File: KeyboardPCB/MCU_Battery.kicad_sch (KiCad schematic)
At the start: 23 parts, among them U1 ATmega32U4-M, U2 TPS61222DCK, U3 MCP73831-2-OT, Y1 ECS-160-7-33B-CKL-TR

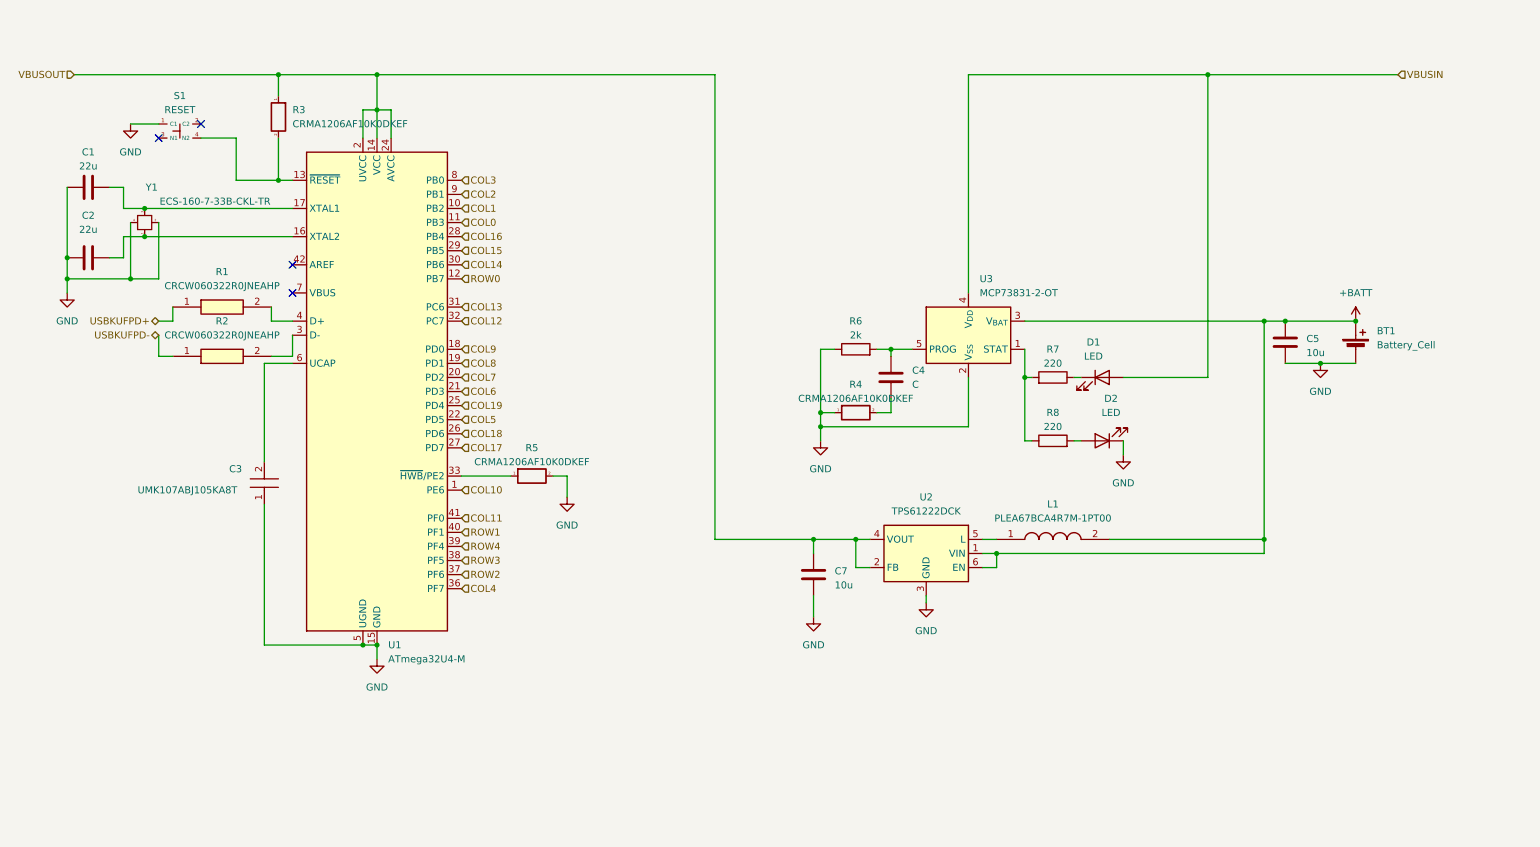
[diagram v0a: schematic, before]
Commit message: changed several components
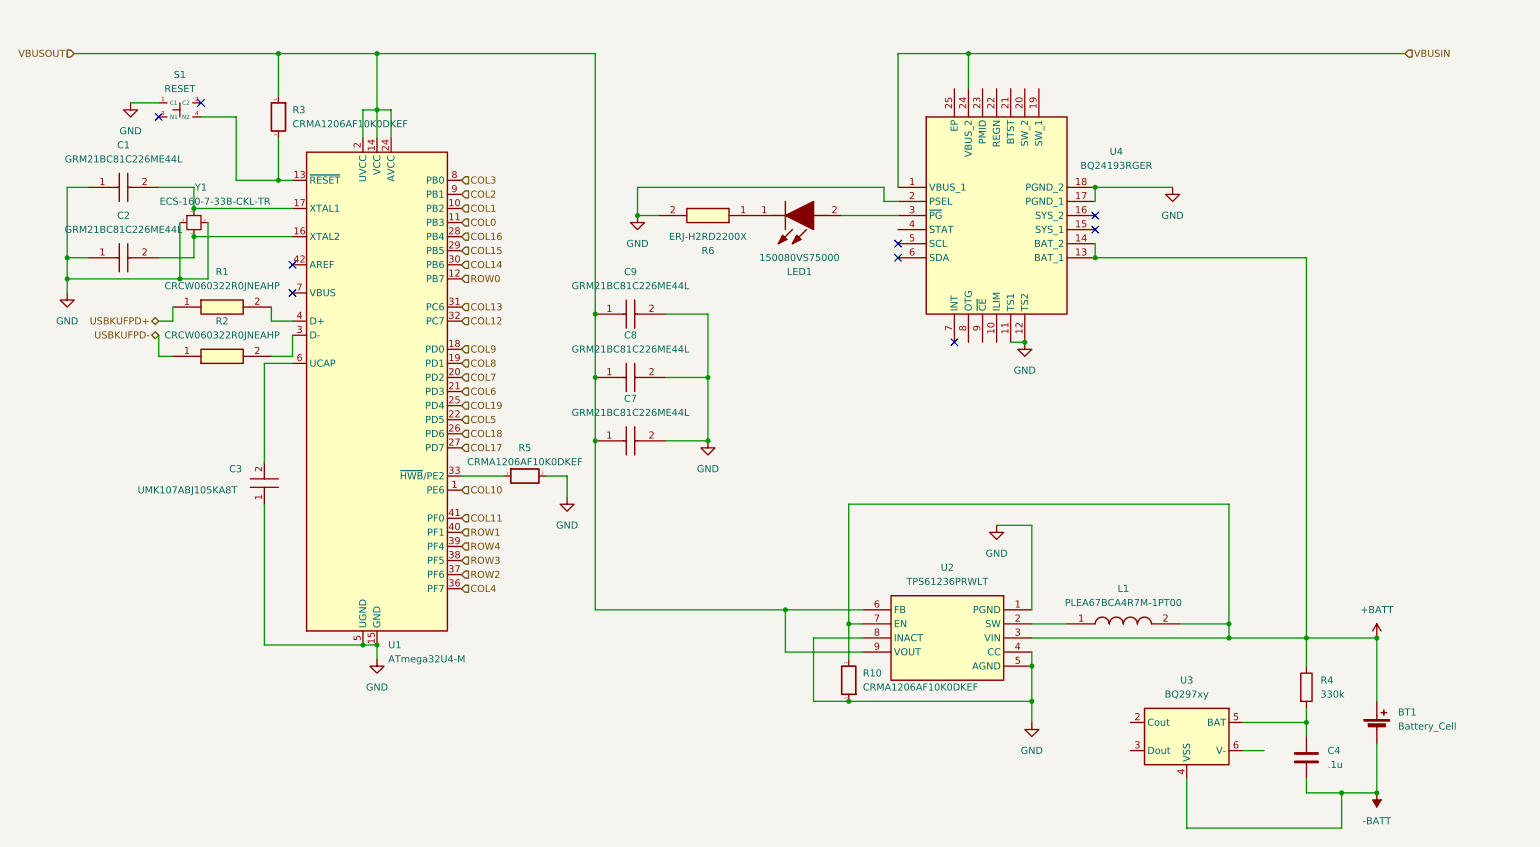
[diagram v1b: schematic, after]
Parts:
- removed C1, C2: 22u, symbol Device:C
- removed C5, C7: 10u, symbol Device:C
- removed D1, D2: LED, symbol Device:LED
- removed R4: CRMA1206AF10K0DKEF, keyboard_syms:RESC3216X74N, symbol keyboard_syms:CRMA1206AF10K0DKEF
- removed R6: 2k, symbol Device:R
- removed R7, R8: 220, symbol Device:R
- removed U2: TPS61222DCK, Package_TO_SOT_SMD:Texas_R-PDSO-G6, symbol Regulator_Switching:TPS61222DCK
- removed U3: MCP73831-2-OT, Package_TO_SOT_SMD:SOT-23-5, symbol Battery_Management:MCP73831-2-OT
- added C1, C2, C7, C8, C9: GRM21BC81C226ME44L, keyboard_syms:CAPC2012X145N, symbol keyboard_syms:GRM21BC81C226ME44L
- added LED1: 150080VS75000, keyboard_syms:LEDC2012X80N, symbol keyboard_syms:150080VS75000
- added R10: CRMA1206AF10K0DKEF, keyboard_syms:RESC3216X74N, symbol keyboard_syms:CRMA1206AF10K0DKEF
- added R4: 330k, symbol Device:R
- added R6: ERJ-H2RD2200X, keyboard_syms:H2C_H2R, symbol keyboard_syms:ERJ-H2RD2200X
- added U2: TPS61236PRWLT, keyboard_syms:TPS61235PRWLT, symbol keyboard_syms:TPS61236PRWLT
- added U3: BQ297xy, Package_SON:WSON-6_1.5x1.5mm_P0.5mm, symbol Battery_Management:BQ297xy
- added U4: BQ24193RGER, keyboard_syms:QFN50P400X400X100-25N-D, symbol keyboard_syms:BQ24193RGER
- C4: value C -> .1u
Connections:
- net +BATT: now also R10.2, R4.1, U2.3 (VIN), U2.7 (EN), U4.13 (BAT_1), U4.14 (BAT_2)
- net GND: now also C1.1, C2.1, C7.2, C8.2, C9.2, R10.1, R6.2, U2.1 (PGND), U2.4 (CC), U2.5 (AGND), U2.8 (INACT), U4.11 (TS1), U4.12 (TS2), U4.17 (PGND_1), U4.18 (PGND_2), U4.2 (PSEL); no longer BT1.2 (-)
- net VBUSIN: now also U4.1 (VBUS_1), U4.24 (VBUS_2)
- net VBUSOUT: now also C7.1, C8.1, C9.1, U2.6 (FB), U2.9 (VOUT)
- net at C4.1: now also R4.2, U3.5 (BAT)
- net -BATT: now reaches C4.2
- net -BATT: now also BT1.2 (-), U3.4 (VSS)
- net at U1.16 (XTAL2), Y1.1: now also C2.2
- net at U1.17 (XTAL1), Y1.3: now also C1.2
- net at L1.1: now also U2.2 (SW)
- new net: LED1.1 (K), R6.1
- new net: LED1.2 (A), U4.3 (~{PG})
- no-connect marks 4 -> 9
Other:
- moved on the sheet: R5, S1, Y1

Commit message: made changes to the board
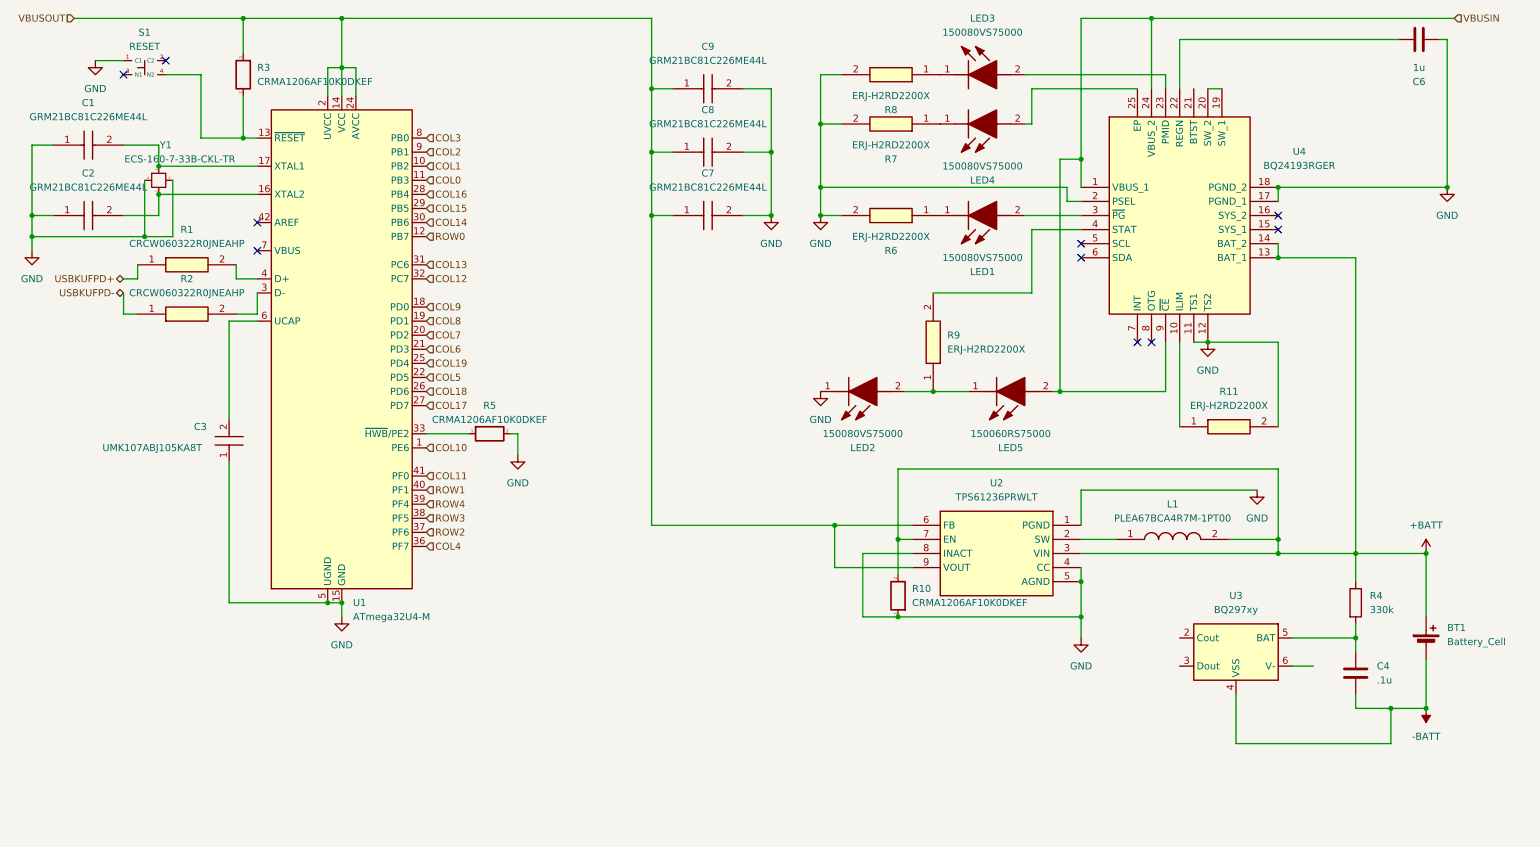
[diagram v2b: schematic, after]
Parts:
- added C6: 1u, symbol Device:C
- added LED2, LED3, LED4: 150080VS75000, keyboard_syms:LEDC2012X80N, symbol keyboard_syms:150080VS75000
- added LED5: 150060RS75000, keyboard_syms:LEDC1608X80N, symbol keyboard_syms:150060RS75000
- added R11, R7, R8, R9: ERJ-H2RD2200X, keyboard_syms:H2C_H2R, symbol keyboard_syms:ERJ-H2RD2200X
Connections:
- net GND: now also C6.2, LED2.1 (K), R11.2, R7.2, R8.2
- net VBUSIN: now also U4.9 (~{CE}), LED5.2 (A)
- net at U4.10 (ILIM): now also R11.1
- net at U4.19 (SW_1): now also U4.20 (SW_2)
- net at U4.22 (REGN): now also C6.1
- net at U4.23 (PMID): now also LED3.2 (A)
- net at U4.25 (EP): now also LED4.2 (A)
- net at U4.4 (STAT): now also R9.2
- new net: LED4.1 (K), R7.1
- new net: LED3.1 (K), R8.1
- new net: LED2.2 (A), LED5.1 (K), R9.1
- no-connect marks 9 -> 10
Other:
- moved on the sheet: BT1, C1, C2, C3, C4, C7, C8, C9, L1, LED1, R1, R10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

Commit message: Schematic Filled out
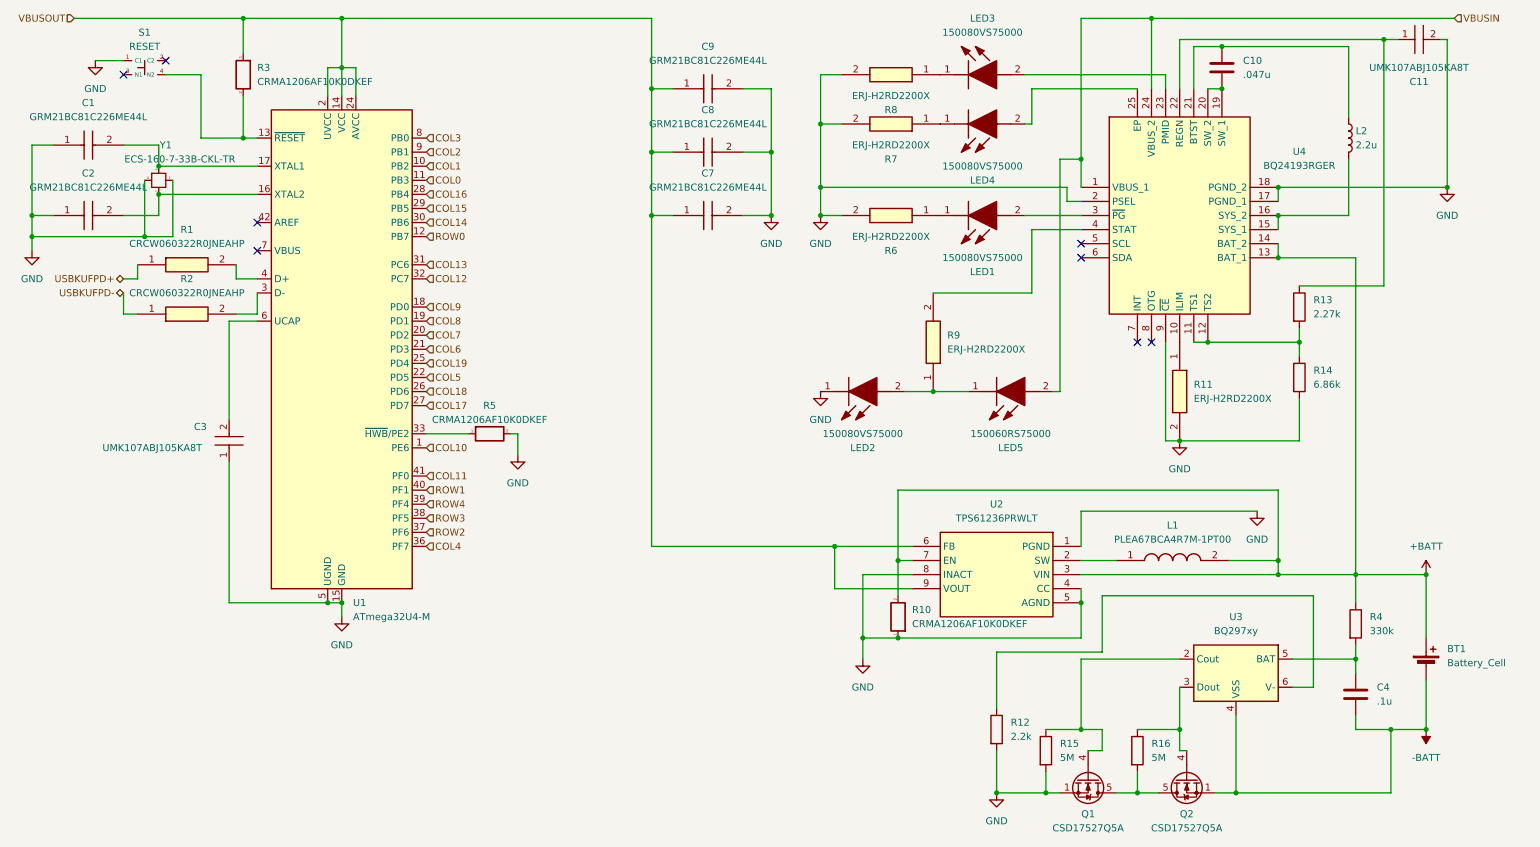
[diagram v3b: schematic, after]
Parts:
- removed C6: 1u, symbol Device:C
- added C10: .047u, symbol Device:C
- added C11: UMK107ABJ105KA8T, keyboard_syms:CAPC1608X95N, symbol keyboard_syms:UMK107ABJ105KA8T
- added L2: 2.2u, symbol Device:L
- added Q1, Q2: CSD17527Q5A, Package_TO_SOT_SMD:TDSON-8-1, symbol Transistor_FET:CSD17527Q5A
- added R12: 2.2k, symbol Device:R
- added R13: 2.27k, symbol Device:R
- added R14: 6.86k, symbol Device:R
- added R15, R16: 5M, symbol Device:R
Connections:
- net -BATT: now also Q2.1 (S), Q2.2 (S), Q2.3 (S)
- net GND: now also U4.9 (~{CE}), C11.2, Q1.1 (S), Q1.2 (S), Q1.3 (S), R12.2, R14.2, R15.2; no longer U4.11 (TS1), U4.12 (TS2)
- net VBUSIN: no longer U4.9 (~{CE})
- net at U3.2 (Cout): now also Q1.4 (G), R15.1
- net at U3.3 (Dout): now also Q2.4 (G), R16.1
- net at U3.6 (V-): now also R12.1
- net at U4.22 (REGN): now also C11.1, R13.1
- net at U4.15 (SYS_1): now also U4.16 (SYS_2), L2.2
- net at U4.19 (SW_1), U4.20 (SW_2): now also C10.2
- net at U4.21 (BTST): now also C10.1, L2.1
- new net: Q1.5 (D), Q2.5 (D), R16.2
- new net: R13.2, R14.1, U4.11 (TS1), U4.12 (TS2)
- no-connect marks 10 -> 8
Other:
- moved on the sheet: BT1, C4, L1, R10, R11, R4, U2, U3
